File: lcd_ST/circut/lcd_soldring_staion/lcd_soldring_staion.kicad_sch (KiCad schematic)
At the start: 43 parts, among them J1 DIN-5, J10 Conn_01x03_Pin, J2 Conn_01x05_Pin, J3 Conn_01x01_Pin, J4 Conn_01x01_Pin, J44 Screw_Terminal_01x02, J5 Conn_01x01_Pin, J6 Conn_01x01_Pin, J7 Conn_01x04_Pin, J8 Conn_01x04_Pin, J9 Conn_01x04_Pin, Q2 Si4162DY, SW1 SW_Push, U1 PIC16F15223T-I/SL, U2 L7805, U3 LM358

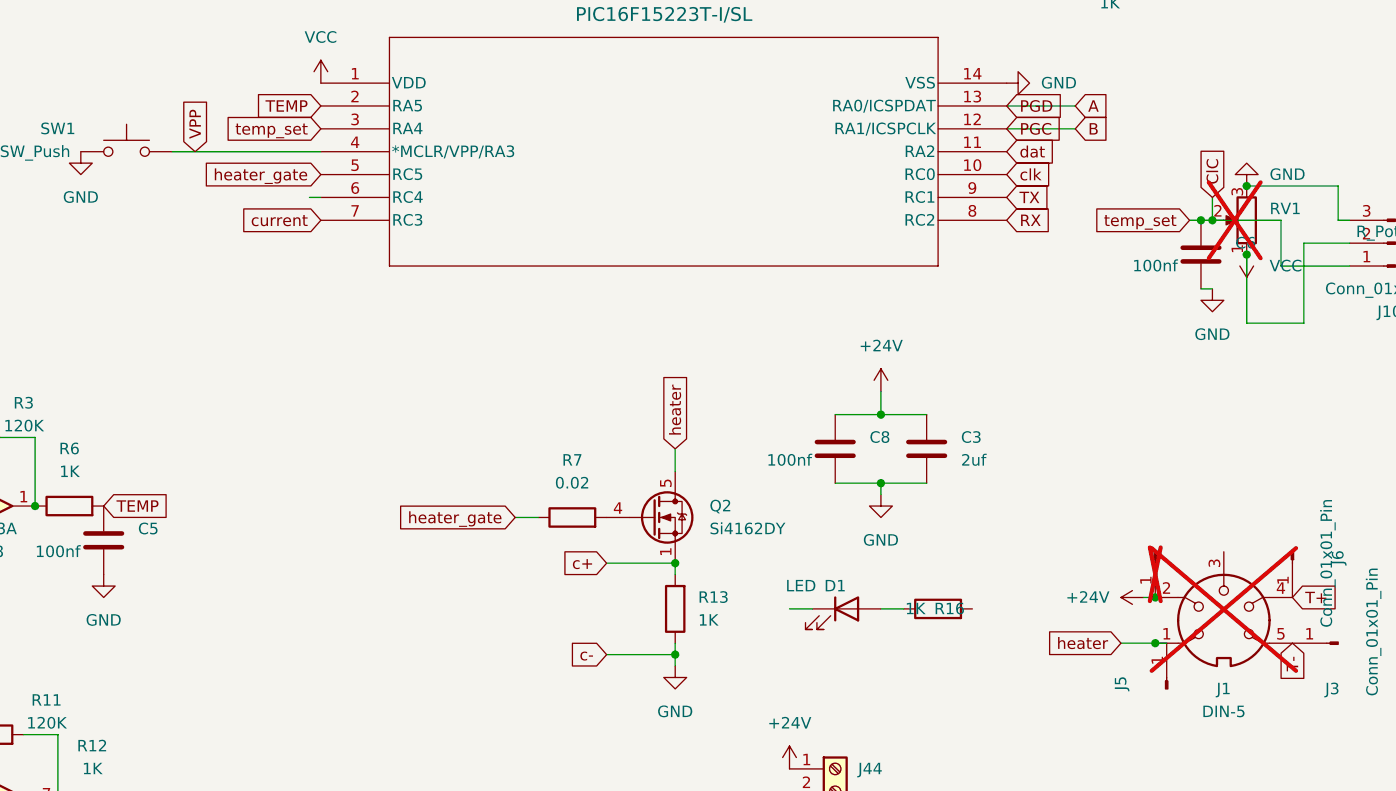
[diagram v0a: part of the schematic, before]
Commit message: h
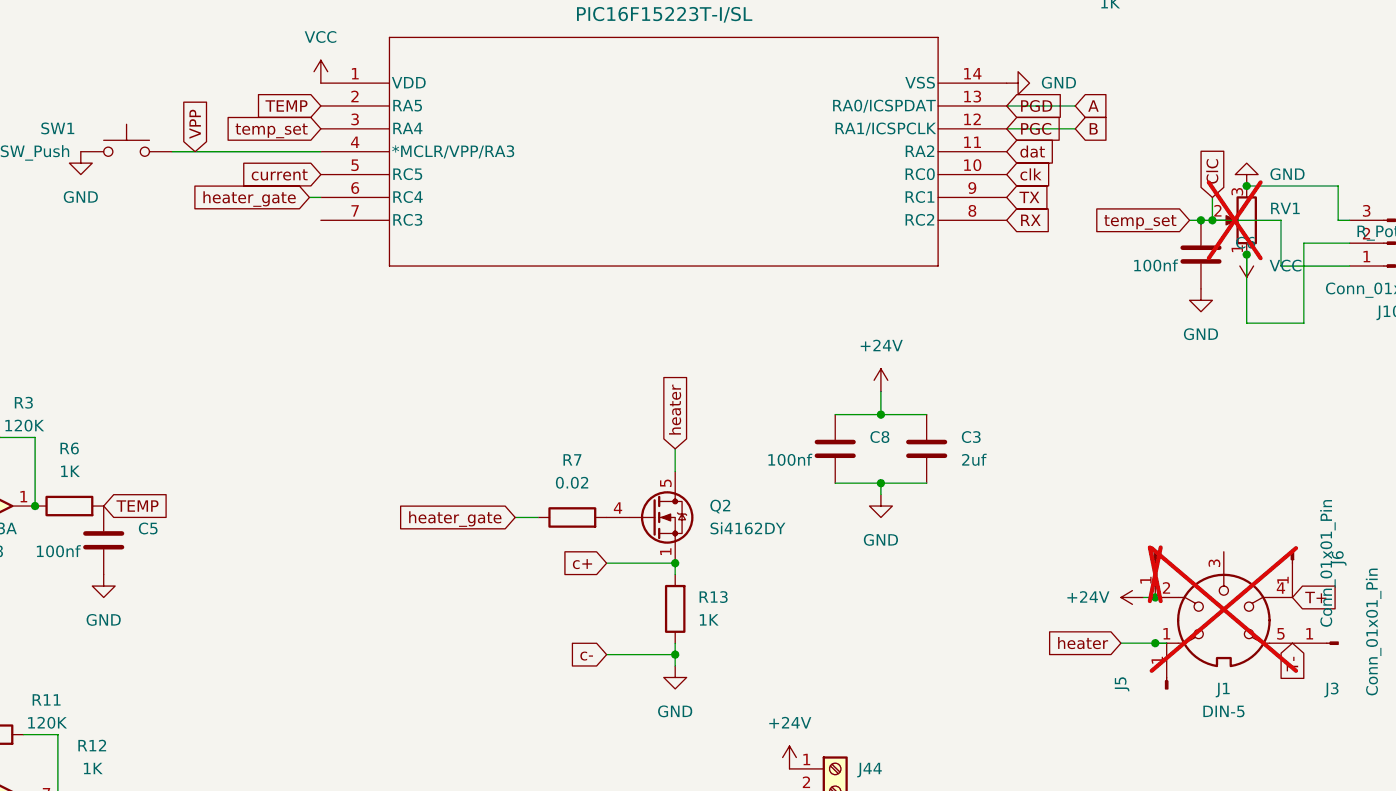
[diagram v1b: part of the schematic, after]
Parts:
- removed D1: LED, LED_SMD:LED_1210_3225Metric_Pad1.42x2.65mm_HandSolder, symbol Device:LED
- removed R16: 1K, Resistor_SMD:R_0805_2012Metric_Pad1.20x1.40mm_HandSolder, symbol Device:R
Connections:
- net current: now also U1.5 (RC5); no longer U1.7 (RC3)
- net heater_gate: now also U1.6 (RC4); no longer U1.5 (RC5)
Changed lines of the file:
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@@
 	(wire
 		(pts
-			(xy 254 96.52) (xy 255.27 96.52)
-		)
-		(stroke
-			(width 0)
-			(type default)
-		)
-	)
-	(wire
-		(pts
 			(xy 41.91 64.77) (xy 43.18 64.77)
 		)
@@
 	(wire
 		(pts
-			(xy 220.98 132.08) (xy 218.44 132.08)
-		)
-		(stroke
-			(width 0)
-			(type default)
-		)
-	)
-	(wire
-		(pts
 			(xy 95.25 157.48) (xy 104.14 157.48)
 		)
@@
 	(wire
 		(pts
-			(xy 208.28 132.08) (xy 210.82 132.08)
-		)
-		(stroke
-			(width 0)
-			(type default)
-		)
-	)
-	(wire
-		(pts
 			(xy 232.41 78.74) (xy 240.03 78.74)
 		)
@@
 		)
 	)
-	(global_label "current"
-		(shape input)
-		(at 156.21 88.9 180)
-		(fields_autoplaced yes)
-		(effects
-			(font
-				(size 1.27 1.27)
-			)
-			(justify right)
-		)
-		(property "Intersheetrefs" "${INTERSHEET_REFS}"
-			(at 146.4515 88.9 0)
-			(effects
-				(font
-					(size 1.27 1.27)
-				)
-				(justify right)
-				(hide yes)
-			)
-		)
-	)
 	(global_label "c-"
 		(shape input)
@@
 		)
 	)
-	(global_label "heater"
+	(global_label "current"
 		(shape input)
-		(at 195.58 114.3 90)
+		(at 156.21 83.82 180)
 		(fields_autoplaced yes)
 		(effects
@@
 				(size 1.27 1.27)
 			)
-			(justify left)
+			(justify right)
 		)
 		(property "Intersheetrefs" "${INTERSHEET_REFS}"
-			(at 195.58 105.3277 90)
+			(at 146.4515 83.82 0)
 			(effects
 				(font
 					(size 1.27 1.27)
 				)
-				(justify left)
+				(justify right)
 				(hide yes)
 			)
 		)
 	)
-	(global_label "B"
+	(global_label "heater"
 		(shape input)
-		(at 240.03 78.74 0)
+		(at 195.58 114.3 90)
 		(fields_autoplaced yes)
 		(effects
@@
 		)
 		(property "Intersheetrefs" "${INTERSHEET_REFS}"
-			(at 244.2852 78.74 0)
+			(at 195.58 105.3277 90)
 			(effects
 				(font
@@
 		)
 	)
-	(global_label "heater_gate"
+	(global_label "B"
 		(shape input)
-		(at 156.21 83.82 180)
+		(at 240.03 78.74 0)
 		(fields_autoplaced yes)
 		(effects
@@
 				(size 1.27 1.27)
 			)
-			(justify right)
+			(justify left)
 		)
 		(property "Intersheetrefs" "${INTERSHEET_REFS}"
-			(at 142.1578 83.82 0)
+			(at 244.2852 78.74 0)
 			(effects
 				(font
 					(size 1.27 1.27)
 				)
-				(justify right)
+				(justify left)
 				(hide yes)
 			)
@@
 		)
 	)
+	(global_label "heater_gate"
+		(shape input)
+		(at 154.94 86.36 180)
+		(fields_autoplaced yes)
+		(effects
+			(font
+				(size 1.27 1.27)
+			)
+			(justify right)
+		)
+		(property "Intersheetrefs" "${INTERSHEET_REFS}"
+			(at 140.8878 86.36 0)
+			(effects
+				(font
+					(size 1.27 1.27)
+				)
+				(justify right)
+				(hide yes)
+			)
+		)
+	)
 	(global_label "temp_set"
 		(shape input)
@@
 	)
 	(symbol
-		(lib_id "Device:R")
-		(at 224.79 132.08 90)
-		(unit 1)
-		(exclude_from_sim no)
-		(in_bom yes)
-		(on_board yes)
-		(dnp no)
-		(property "Reference" "R16"
-			(at 226.06 132.08 90)
-			(effects
-				(font
-					(size 1.27 1.27)
-				)
-			)
-		)
-		(property "Value" "1K"
-			(at 222.25 132.08 90)
-			(effects
-				(font
-					(size 1.27 1.27)
-				)
-			)
-		)
-		(property "Footprint" "Resistor_SMD:R_0805_2012Metric_Pad1.20x1.40mm_HandSolder"
-			(at 224.79 133.858 90)
-			(effects
-				(font
-					(size 1.27 1.27)
-				)
-				(hide yes)
-			)
-		)
-		(property "Datasheet" "~"
-			(at 224.79 132.08 0)
-			(effects
-				(font
-					(size 1.27 1.27)
-				)
-				(hide yes)
-			)
-		)
-		(property "Description" "Resistor"
-			(at 224.79 132.08 0)
-			(effects
-				(font
-					(size 1.27 1.27)
-				)
-				(hide yes)
-			)
-		)
-		(pin "1"
-		)
-		(pin "2"
-		)
-		(instances
-			(project "lcd_soldring_staion"
-				(path "/0f7f1c9d-acb7-4f35-a7f1-2d89c4552cf7"
-					(reference "R16")
-					(unit 1)
-				)
-			)
-		)
-	)
-	(symbol
 		(lib_id "power:GND")
 		(at 275.59 22.86 90)
@@
 	)
 	(symbol
-		(lib_id "Device:LED")
-		(at 214.63 132.08 0)
-		(unit 1)
-		(exclude_from_sim no)
-		(in_bom yes)
-		(on_board yes)
-		(dnp no)
-		(property "Reference" "D1"
-			(at 213.36 129.54 0)
-			(effects
-				(font
-					(size 1.27 1.27)
-				)
-			)
-		)
-		(property "Value" "LED"
-			(at 209.55 129.54 0)
-			(effects
-				(font
-					(size 1.27 1.27)
-				)
-			)
-		)
-		(property "Footprint" "LED_SMD:LED_1210_3225Metric_Pad1.42x2.65mm_HandSolder"
-			(at 214.63 132.08 0)
-			(effects
-				(font
-					(size 1.27 1.27)
-				)
-				(hide yes)
-			)
-		)
-		(property "Datasheet" "~"
-			(at 214.63 132.08 0)
-			(effects
-				(font
-					(size 1.27 1.27)
-				)
-				(hide yes)
-			)
-		)
-		(property "Description" "Light emitting diode"
-			(at 214.63 132.08 0)
-			(effects
-				(font
-					(size 1.27 1.27)
-				)
-				(hide yes)
-			)
-		)
-		(property "Sim.Pins" "1=K 2=A"
-			(at 214.63 132.08 0)
-			(effects
-				(font
-					(size 1.27 1.27)
-				)
-				(hide yes)
-			)
-		)
-		(pin "2"
-		)
-		(pin "1"
-		)
-		(instances
-			(project "lcd_soldring_staion"
-				(path "/0f7f1c9d-acb7-4f35-a7f1-2d89c4552cf7"
-					(reference "D1")
-					(unit 1)
-				)
-			)
-		)
-	)
-	(symbol
 		(lib_id "Device:C")
 		(at 223.52 114.3 0)
@@
 	(symbol
 		(lib_id "power:GND")
-		(at 255.27 96.52 0)
+		(at 254 96.52 0)
 		(unit 1)
 		(exclude_from_sim no)
@@
 		(fields_autoplaced yes)
 		(property "Reference" "#PWR023"
-			(at 255.27 102.87 0)
+			(at 254 102.87 0)
 			(effects
 				(font
@@
 		)
 		(property "Value" "GND"
-			(at 255.27 101.6 0)
+			(at 254 101.6 0)
 			(effects
 				(font
@@
 		)
 		(property "Footprint" ""
-			(at 255.27 96.52 0)
+			(at 254 96.52 0)
 			(effects
 				(font
@@
 		)
 		(property "Datasheet" ""
-			(at 255.27 96.52 0)
+			(at 254 96.52 0)
 			(effects
 				(font
@@
 		)
 		(property "Description" "Power symbol creates a global label with name \"GND\" , ground"
-			(at 255.27 96.52 0)
+			(at 254 96.52 0)
 			(effects
 				(font

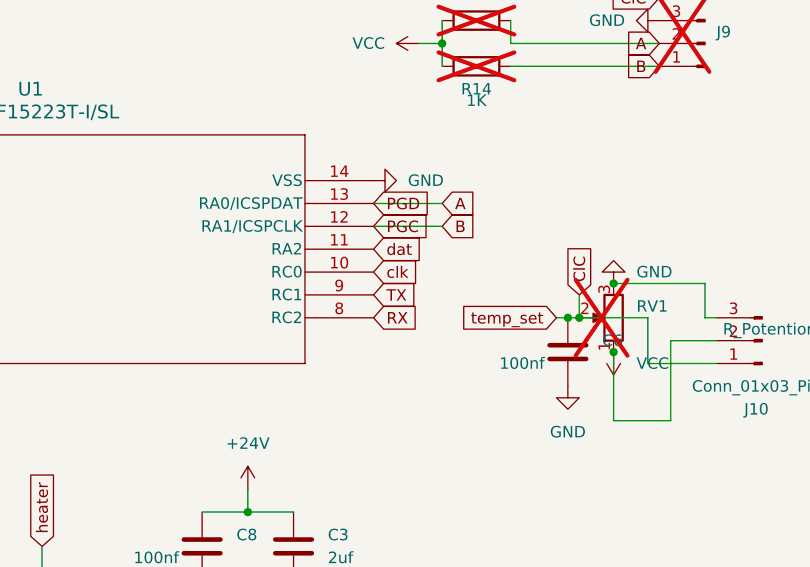
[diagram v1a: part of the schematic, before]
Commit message: final_final
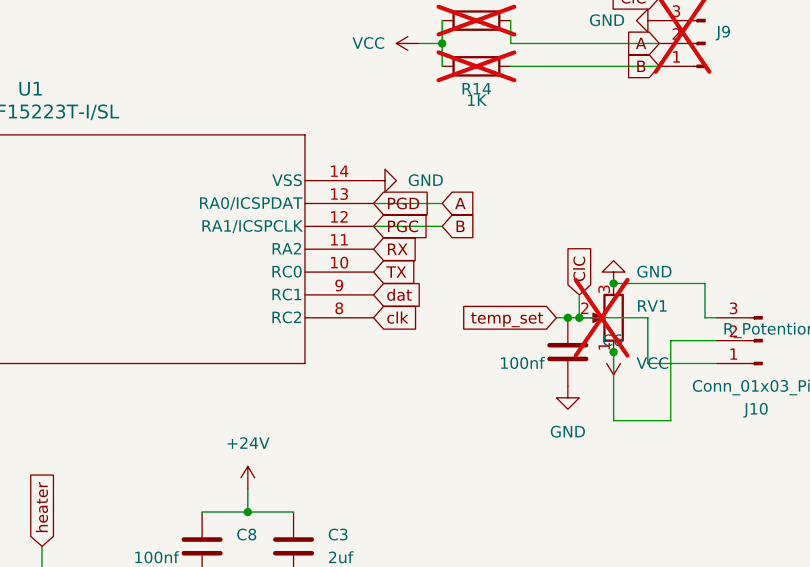
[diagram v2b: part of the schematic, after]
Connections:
- net RX: now also U1.11 (RA2); no longer U1.8 (RC2)
- net TX: now also U1.10 (RC0); no longer U1.9 (RC1)
- net clk: now also U1.8 (RC2); no longer U1.10 (RC0)
- net dat: now also U1.9 (RC1); no longer U1.11 (RA2)
